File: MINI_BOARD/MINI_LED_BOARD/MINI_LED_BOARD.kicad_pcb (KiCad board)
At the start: 2 copper layers, 35 parts, among them J1 Conn_ARM_SWD_TagConnect_TC2030, J2 430450428, U1 MSPM0C1103SDDFR, U4 TPS76333DBVR

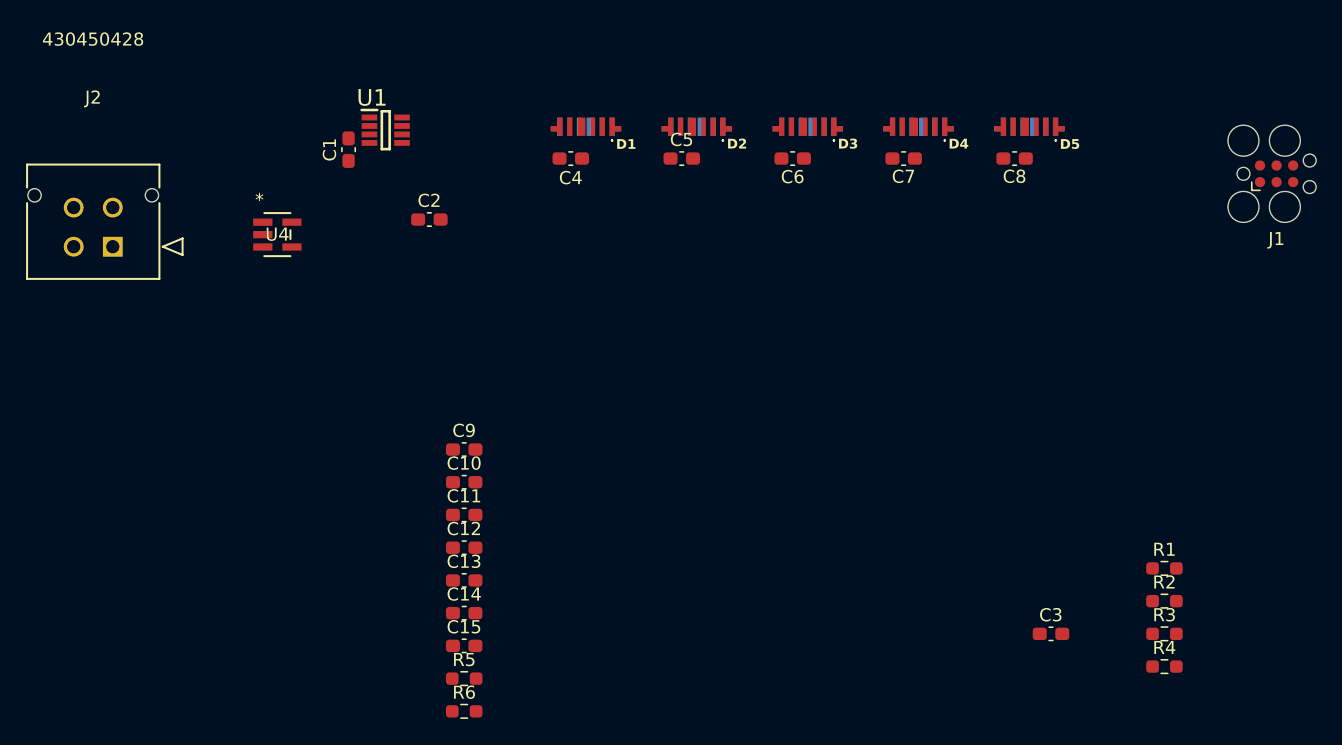
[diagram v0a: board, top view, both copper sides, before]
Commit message: Complete more major layout placement
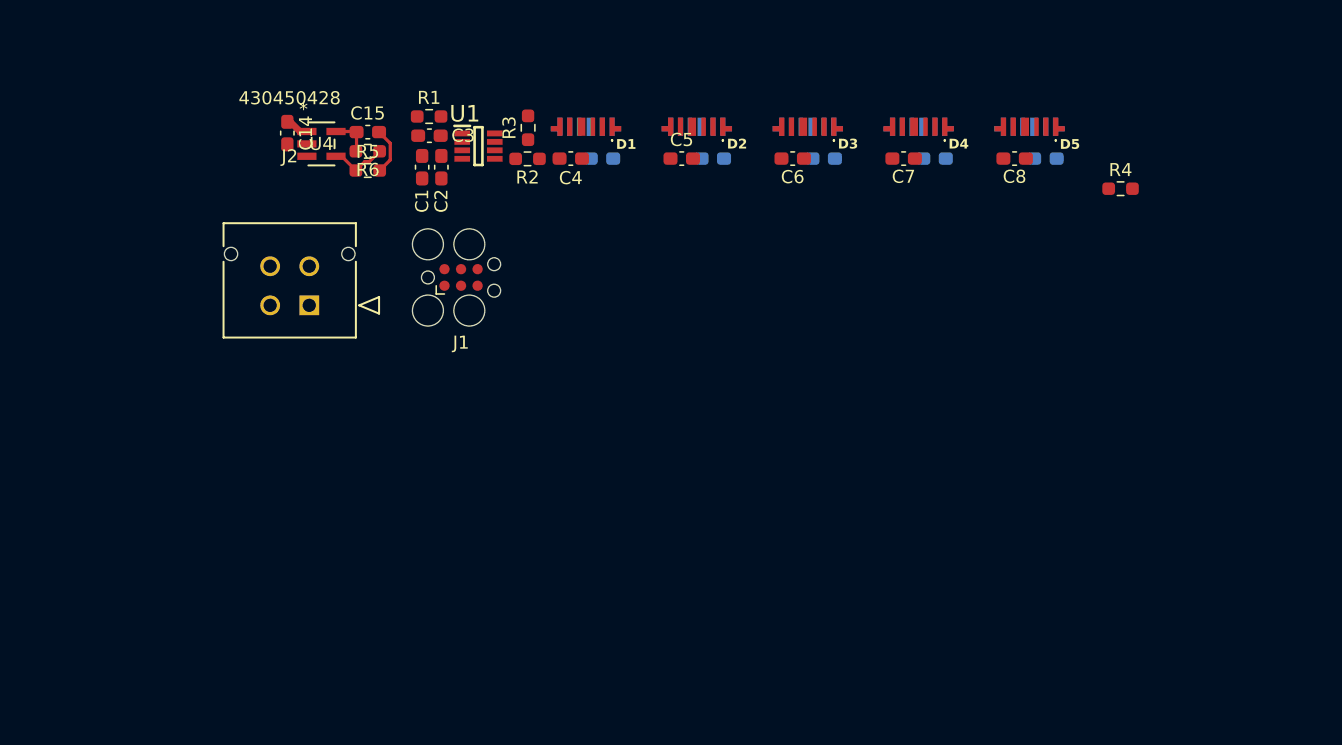
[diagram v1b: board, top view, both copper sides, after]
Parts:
- C10, C11, C12, C13, C9: moved to B.Cu
- moved R1 66.2 mm to (70.6, 54.5)
- moved J1 63.0 mm to (73.0, 66.8)
- moved R3 62.4 mm to (78.2, 55.3), turned to 90 degrees
- moved C3 61.1 mm to (70.6, 55.9), turned to 180 degrees
- moved R2 59.5 mm to (78.1, 57.7), turned to 180 degrees
- moved C13 55.1 mm to (117.9, 57.7), turned to 180 degrees
- moved C12 46.8 mm to (109.4, 57.7), turned to 180 degrees
- moved R6 43.6 mm to (65.9, 57.1), turned to 180 degrees
- moved C15 40.1 mm to (65.9, 55.7)
- moved R5 39.7 mm to (65.9, 58.6)
- moved C14 39.2 mm to (59.7, 55.7), turned to -90 degrees
- moved C11 38.8 mm to (100.8, 57.7), turned to 180 degrees
- moved R4 36.8 mm to (123.6, 60.0)
- moved C10 31.3 mm to (92.3, 57.7), turned to 180 degrees
- moved C9 24.7 mm to (83.8, 57.7), turned to 180 degrees
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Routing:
- net Net-(U4-NC/FB): track 0.00 -> 4.41 mm
- net GND: track 0.00 -> 3.64 mm
- net +3.3V: track 0.00 -> 3.09 mm
- net +5V: track 0.00 -> 1.81 mm
